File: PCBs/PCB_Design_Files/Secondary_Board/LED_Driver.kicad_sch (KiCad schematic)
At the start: 14 parts, among them Q1 MMBT3904, Q2 MMBT3904, Q5 2N7002, Q6 BSS84, Q7 2N7002, Q8 BSS84, U8 OPA333AIDCKR

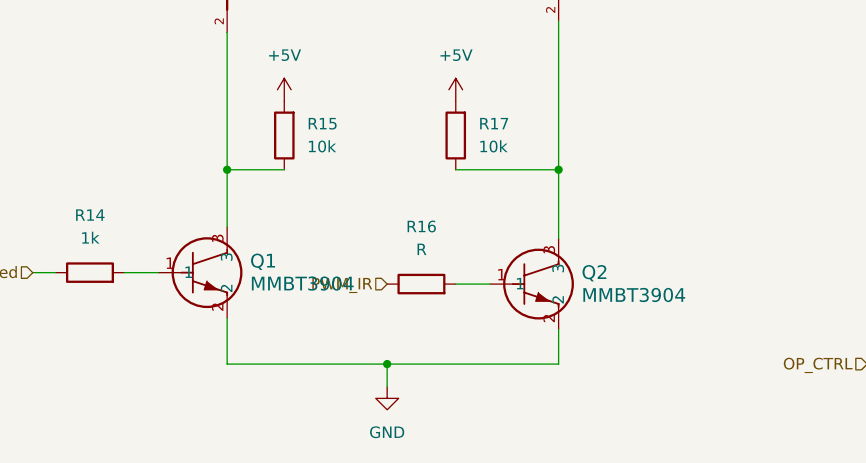
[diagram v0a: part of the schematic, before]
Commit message: BOM updated
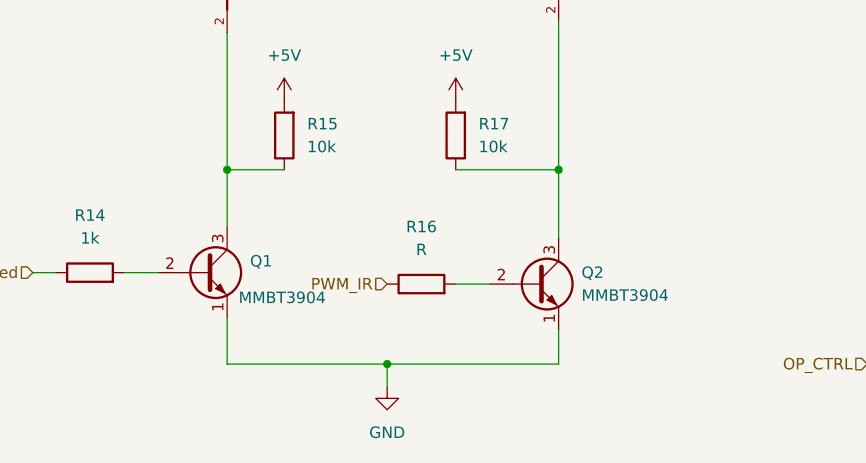
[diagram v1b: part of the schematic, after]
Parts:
- removed Q1, Q2: MMBT3904, Project Footprints:SOT23_FAS, symbol Project_Symbols:MMBT3904
- added Q1, Q2: MMBT3904, Package_TO_SOT_SMD:SOT-23, symbol Transistor_BJT:2N3904
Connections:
- net GND: now also Q1.1 (E), Q2.1 (E)
- net at R14.2: now also Q1.2 (B)
- net at Q6.2 (S), R15.1: now also Q1.3 (C)
- net at R16.2: now also Q2.2 (B)
- net at Q8.2 (S), R17.1: now also Q2.3 (C)
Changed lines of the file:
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@@
+	)
+	(symbol
+		(lib_id "Transistor_BJT:2N3904")
+		(at 96.52 127 0)
+		(unit 1)
+		(exclude_from_sim no)
+		(in_bom yes)
+		(on_board yes)
+		(dnp no)
+		(property "Reference" "Q1"
+			(at 101.6 125.7299 0)
+			(effects
+				(font
+					(size 1.27 1.27)
+				)
+				(justify left)
+			)
+		)
+		(property "Value" "MMBT3904"
+			(at 100.33 129.794 0)
+			(effects
+				(font
+					(size 1.27 1.27)
+				)
+				(justify left)
+			)
+		)
+		(property "Footprint" "Package_TO_SOT_SMD:SOT-23"
+			(at 101.6 128.905 0)
+			(effects
+				(font
+					(size 1.27 1.27)
+					(italic yes)
+				)
+				(justify left)
+				(hide yes)
+			)
+		)
+		(property "Datasheet" "https://www.onsemi.com/pub/Collateral/2N3903-D.PDF"
+			(at 96.52 127 0)
+			(effects
+				(font
+					(size 1.27 1.27)
+				)
+				(justify left)
+				(hide yes)
+			)
+		)
+		(property "Description" "0.2A Ic, 40V Vce, Small Signal NPN Transistor, TO-92"
+			(at 96.52 127 0)
+			(effects
+				(font
+					(size 1.27 1.27)
+				)
+				(hide yes)
+			)
+		)
+		(pin "2"
+		)
+		(pin "3"
+		)
+		(pin "1"
+		)
+		(instances
+			(project "Secondary_Board"
+				(path "/2f5986e4-77b2-4f5d-ab91-80ba6228eb8b/16ecf950-1853-427b-9137-65792483b2a5"
+					(reference "Q1")
+					(unit 1)
+				)
+			)
+			(project ""
+				(path "/ed36e940-b5c2-4fa7-8175-f729e6b712de"
+					(reference "Q1")
+					(unit 1)
+				)
+			)
+		)
 	)
 	(symbol
@@
 	)
 	(symbol
-		(lib_id "Project_Symbols:MMBT3904")
-		(at 91.44 127 0)
-		(unit 1)
-		(exclude_from_sim no)
-		(in_bom yes)
-		(on_board yes)
-		(dnp no)
-		(fields_autoplaced yes)
-		(property "Reference" "Q1"
-			(at 101.6 125.7299 0)
-			(effects
-				(font
-					(size 1.524 1.524)
-				)
-				(justify left)
-			)
-		)
-		(property "Value" "MMBT3904"
-			(at 101.6 128.2699 0)
-			(effects
-				(font
-					(size 1.524 1.524)
-				)
-				(justify left)
-			)
-		)
-		(property "Footprint" "Project Footprints:SOT23_FAS"
-			(at 88.9 133.604 0)
-			(effects
-				(font
-					(size 1.27 1.27)
-					(italic yes)
-				)
-				(hide yes)
-			)
-		)
-		(property "Datasheet" "MMBT3904"
-			(at 88.9 133.604 0)
-			(effects
-				(font
-					(size 1.27 1.27)
-					(italic yes)
-				)
-				(hide yes)
-			)
-		)
-		(property "Description" ""
-			(at 91.44 127 0)
-			(effects
-				(font
-					(size 1.27 1.27)
-				)
-				(hide yes)
-			)
-		)
-		(pin "1"
-		)
-		(pin "2"
-		)
-		(pin "3"
-		)
-		(instances
-			(project ""
-				(path "/2f5986e4-77b2-4f5d-ab91-80ba6228eb8b/16ecf950-1853-427b-9137-65792483b2a5"
-					(reference "Q1")
-					(unit 1)
-				)
-			)
-		)
-	)
-	(symbol
 		(lib_id "Device:R")
 		(at 120.65 128.27 90)
@@
 	)
 	(symbol
+		(lib_id "Transistor_BJT:2N3904")
+		(at 133.35 128.27 0)
+		(unit 1)
+		(exclude_from_sim no)
+		(in_bom yes)
+		(on_board yes)
+		(dnp no)
+		(fields_autoplaced yes)
+		(property "Reference" "Q2"
+			(at 138.43 126.9999 0)
+			(effects
+				(font
+					(size 1.27 1.27)
+				)
+				(justify left)
+			)
+		)
+		(property "Value" "MMBT3904"
+			(at 138.43 129.5399 0)
+			(effects
+				(font
+					(size 1.27 1.27)
+				)
+				(justify left)
+			)
+		)
+		(property "Footprint" "Package_TO_SOT_SMD:SOT-23"
+			(at 138.43 130.175 0)
+			(effects
+				(font
+					(size 1.27 1.27)
+					(italic yes)
+				)
+				(justify left)
+				(hide yes)
+			)
+		)
+		(property "Datasheet" "https://www.onsemi.com/pub/Collateral/2N3903-D.PDF"
+			(at 133.35 128.27 0)
+			(effects
+				(font
+					(size 1.27 1.27)
+				)
+				(justify left)
+				(hide yes)
+			)
+		)
+		(property "Description" "0.2A Ic, 40V Vce, Small Signal NPN Transistor, TO-92"
+			(at 133.35 128.27 0)
+			(effects
+				(font
+					(size 1.27 1.27)
+				)
+				(hide yes)
+			)
+		)
+		(pin "3"
+		)
+		(pin "2"
+		)
+		(pin "1"
+		)
+		(instances
+			(project "Secondary_Board"
+				(path "/2f5986e4-77b2-4f5d-ab91-80ba6228eb8b/16ecf950-1853-427b-9137-65792483b2a5"
+					(reference "Q2")
+					(unit 1)
+				)
+			)
+			(project ""
+				(path "/ed36e940-b5c2-4fa7-8175-f729e6b712de"
+					(reference "Q2")
+					(unit 1)
+				)
+			)
+		)
+	)
+	(symbol
 		(lib_id "Project_Symbols:2N7002")
 		(at 179.07 74.93 0)
@@
 					(unit 1)
 				)
-			)
-		)
-	)
-	(symbol
-		(lib_id "Project_Symbols:MMBT3904")
-		(at 128.27 128.27 0)
-		(unit 1)
-		(exclude_from_sim no)
-		(in_bom yes)
-		(on_board yes)
-		(dnp no)
-		(fields_autoplaced yes)
-		(property "Reference" "Q2"
-			(at 138.43 126.9999 0)
-			(effects
-				(font
-					(size 1.524 1.524)
-				)
-				(justify left)
-			)
-		)
-		(property "Value" "MMBT3904"
-			(at 138.43 129.5399 0)
-			(effects
-				(font
-					(size 1.524 1.524)
-				)
-				(justify left)
-			)
-		)
-		(property "Footprint" "Project Footprints:SOT23_FAS"
-			(at 125.73 134.874 0)
-			(effects
-				(font
-					(size 1.27 1.27)
-					(italic yes)
-				)
-				(hide yes)
-			)
-		)
-		(property "Datasheet" "MMBT3904"
-			(at 125.73 134.874 0)
-			(effects
-				(font
-					(size 1.27 1.27)
-					(italic yes)
-				)
-				(hide yes)
-			)
-		)
-		(property "Description" ""
-			(at 128.27 128.27 0)
-			(effects
-				(font
-					(size 1.27 1.27)
-				)
-				(hide yes)
-			)
-		)
-		(pin "1"
-		)
-		(pin "3"
-		)
-		(pin "2"
-		)
-		(instances
-			(project ""
-				(path "/2f5986e4-77b2-4f5d-ab91-80ba6228eb8b/16ecf950-1853-427b-9137-65792483b2a5"
-					(reference "Q2")
-					(unit 1)
-				)
